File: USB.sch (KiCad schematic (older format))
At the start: 13 parts, among them J2 USB_C_Receptacle, U2 CP2102

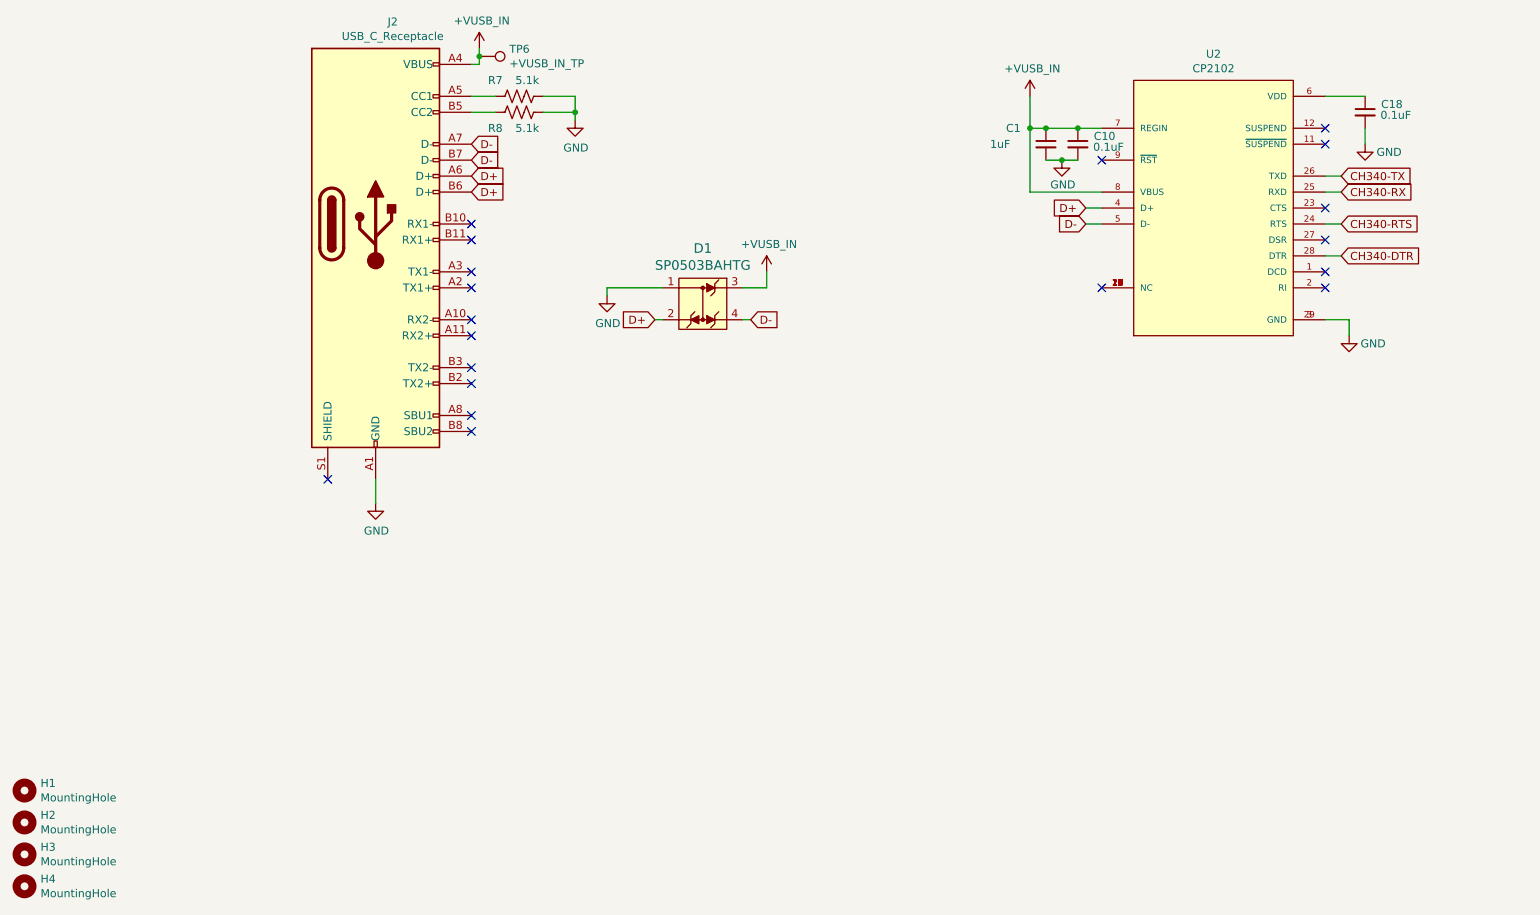
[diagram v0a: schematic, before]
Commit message: Update board
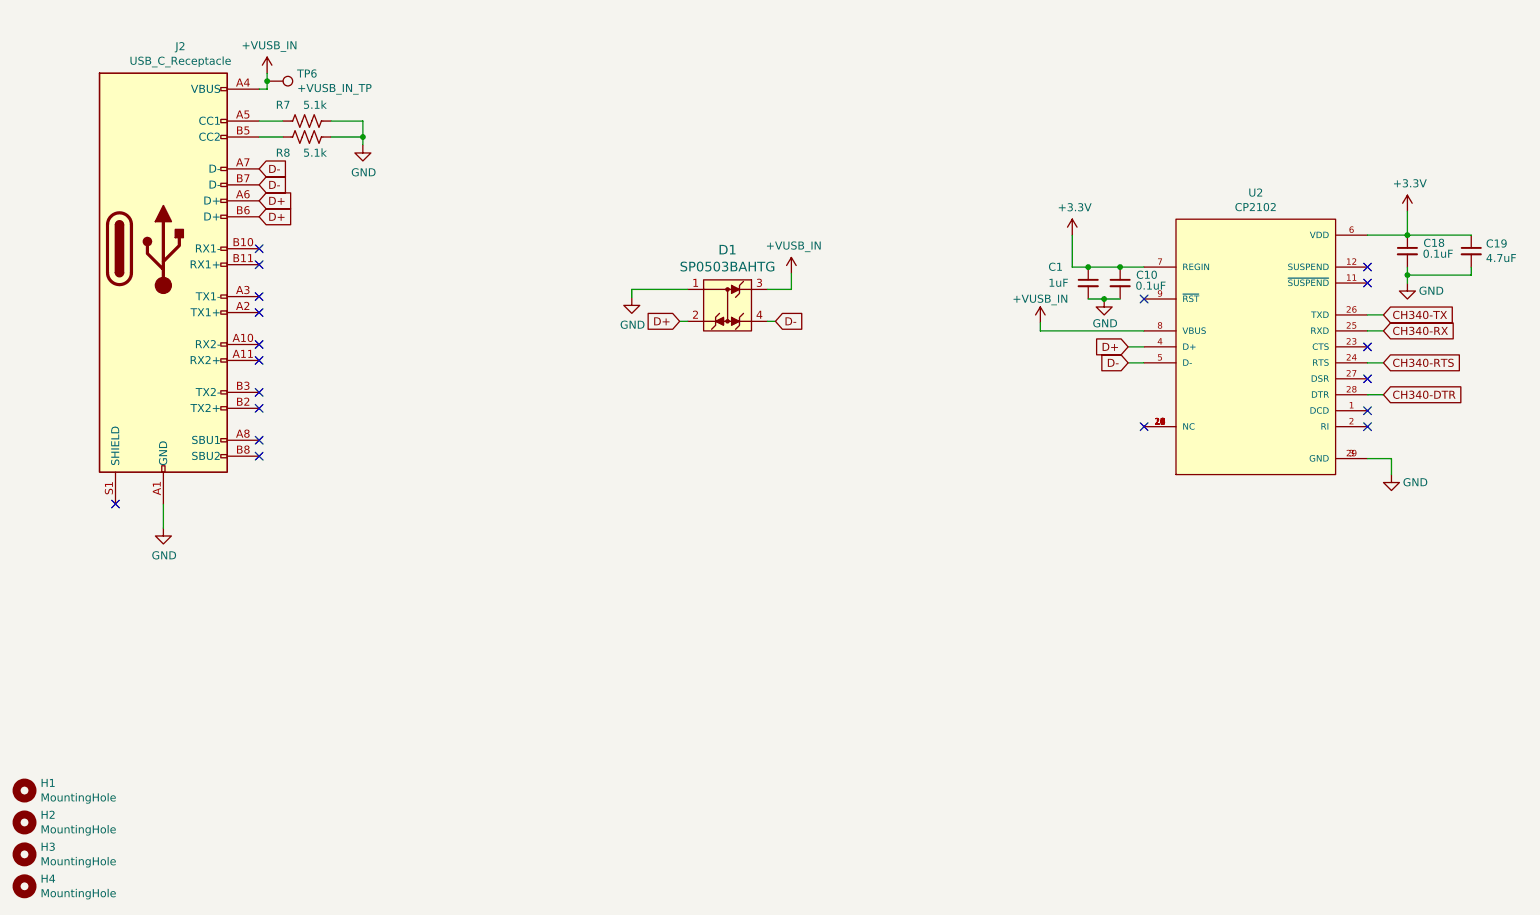
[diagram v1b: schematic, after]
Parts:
- added C19: 4.7uF, Capacitor_SMD:C_0805_2012Metric, symbol Device:C_Small
- C1: footprint (none) -> Capacitor_SMD:C_0603_1608Metric; DigiKey (none) -> https://www.digikey.com/en/products/detail/kemet/C0603C105K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
- C10, C18: DigiKey (none) -> https://www.digikey.com/en/products/detail/kemet/C0603C104J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
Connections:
- net +VUSB_IN: no longer C1.1, C10.1, U2.7 (REGIN)
- net GND: now also C19.2
- net +3V3: now reaches C18.1, U2.6 (VDD)
- net +3V3: now also C1.1, C10.1, U2.7 (REGIN), C19.1
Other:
- moved on the sheet: C1, C10, C18, D1, J2, R7, R8, TP6, U2
